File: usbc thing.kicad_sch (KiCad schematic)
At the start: 15 parts, among them J1 USB_C_Receptacle_USB2.0_16P, Q1 NMOS, U1 P26744EAATRHBRQ1, U4 TPD4S480RUKR

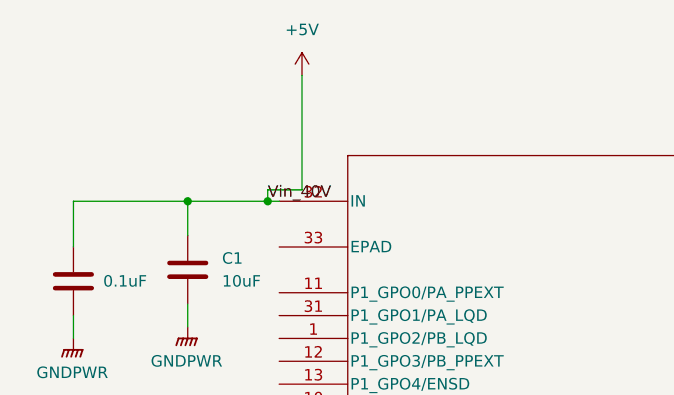
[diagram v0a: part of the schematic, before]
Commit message: changes after 2-26 work meeting
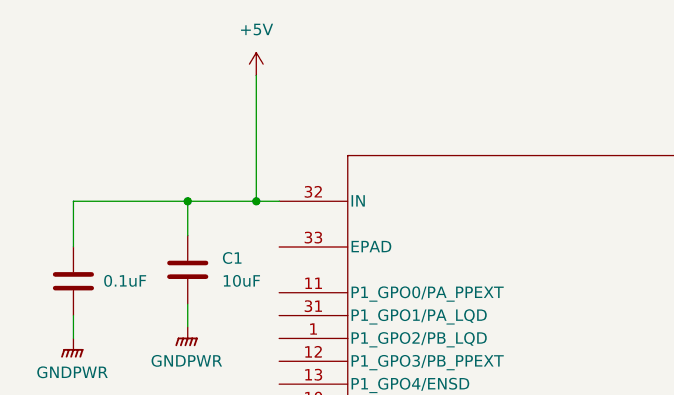
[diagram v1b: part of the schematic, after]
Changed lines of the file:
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@@
+	)
+	(junction
+		(at 40.64 40.64)
+		(diameter 0)
+		(color 0 0 0 0)
 	)
 	(junction
@@
 	)
 	(junction
-		(at 41.91 40.64)
-		(diameter 0)
-		(color 0 0 0 0)
-	)
-	(junction
 		(at 148.59 177.8)
 		(diameter 0)
@@
 	(wire
 		(pts
-			(xy 43.18 40.64) (xy 41.91 40.64)
+			(xy 33.02 40.64) (xy 40.64 40.64)
 		)
 		(stroke
@@
 	(wire
 		(pts
+			(xy 40.64 40.64) (xy 43.18 40.64)
+		)
+		(stroke
+			(width 0)
+			(type default)
+		)
+	)
+	(wire
+		(pts
 			(xy 24.13 73.66) (xy 33.02 73.66)
 		)
@@
 	(wire
 		(pts
-			(xy 41.91 39.37) (xy 41.91 40.64)
-		)
-		(stroke
-			(width 0)
-			(type default)
-		)
-	)
-	(wire
-		(pts
 			(xy 170.18 45.72) (xy 173.99 45.72)
 		)
@@
 	(wire
 		(pts
-			(xy 41.91 40.64) (xy 33.02 40.64)
-		)
-		(stroke
-			(width 0)
-			(type default)
-		)
-	)
-	(wire
-		(pts
-			(xy 41.91 39.37) (xy 45.72 39.37)
-		)
-		(stroke
-			(width 0)
-			(type default)
-		)
-	)
-	(wire
-		(pts
 			(xy 129.54 125.73) (xy 179.07 125.73)
 		)
@@
 	(wire
 		(pts
-			(xy 45.72 39.37) (xy 45.72 26.67)
+			(xy 40.64 26.67) (xy 40.64 40.64)
 		)
 		(stroke
@@
 	(label "SDA"
 		(at 38.1 68.58 0)
-		(effects
-			(font
-				(size 1.27 1.27)
-			)
-			(justify left bottom)
-		)
-	)
-	(label "Vin_40V"
-		(at 41.91 40.64 0)
 		(effects
 			(font
@@
 	(symbol
 		(lib_id "power:+5V")
-		(at 45.72 26.67 0)
+		(at 40.64 26.67 0)
 		(unit 1)
 		(exclude_from_sim no)
@@
 		(fields_autoplaced yes)
 		(property "Reference" "#PWR02"
-			(at 45.72 30.48 0)
+			(at 40.64 30.48 0)
 			(effects
 				(font
@@
 		)
 		(property "Value" "+5V"
-			(at 45.72 21.59 0)
+			(at 40.64 21.59 0)
 			(effects
 				(font
@@
 		)
 		(property "Footprint" ""
-			(at 45.72 26.67 0)
+			(at 40.64 26.67 0)
 			(effects
 				(font
@@
 		)
 		(property "Datasheet" ""
-			(at 45.72 26.67 0)
+			(at 40.64 26.67 0)
 			(effects
 				(font
@@
 		)
 		(property "Description" "Power symbol creates a global label with name \"+5V\""
-			(at 45.72 26.67 0)
-			(effects
-				(font
+			(at 40.64 26.67 0)
+			(effects
+				(font
